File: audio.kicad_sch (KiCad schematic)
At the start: 59 parts, among them IC1 TAC5212IRGER, J13 Headphones 3.5mm, J16 Debug, J18 Jack 6.35mm, J19 Jack 6.35mm, J20 Jack 6.35mm, J22 Jack 6.35mm, U14 OPA1656ID, U7 74AHCT1G32SE-7

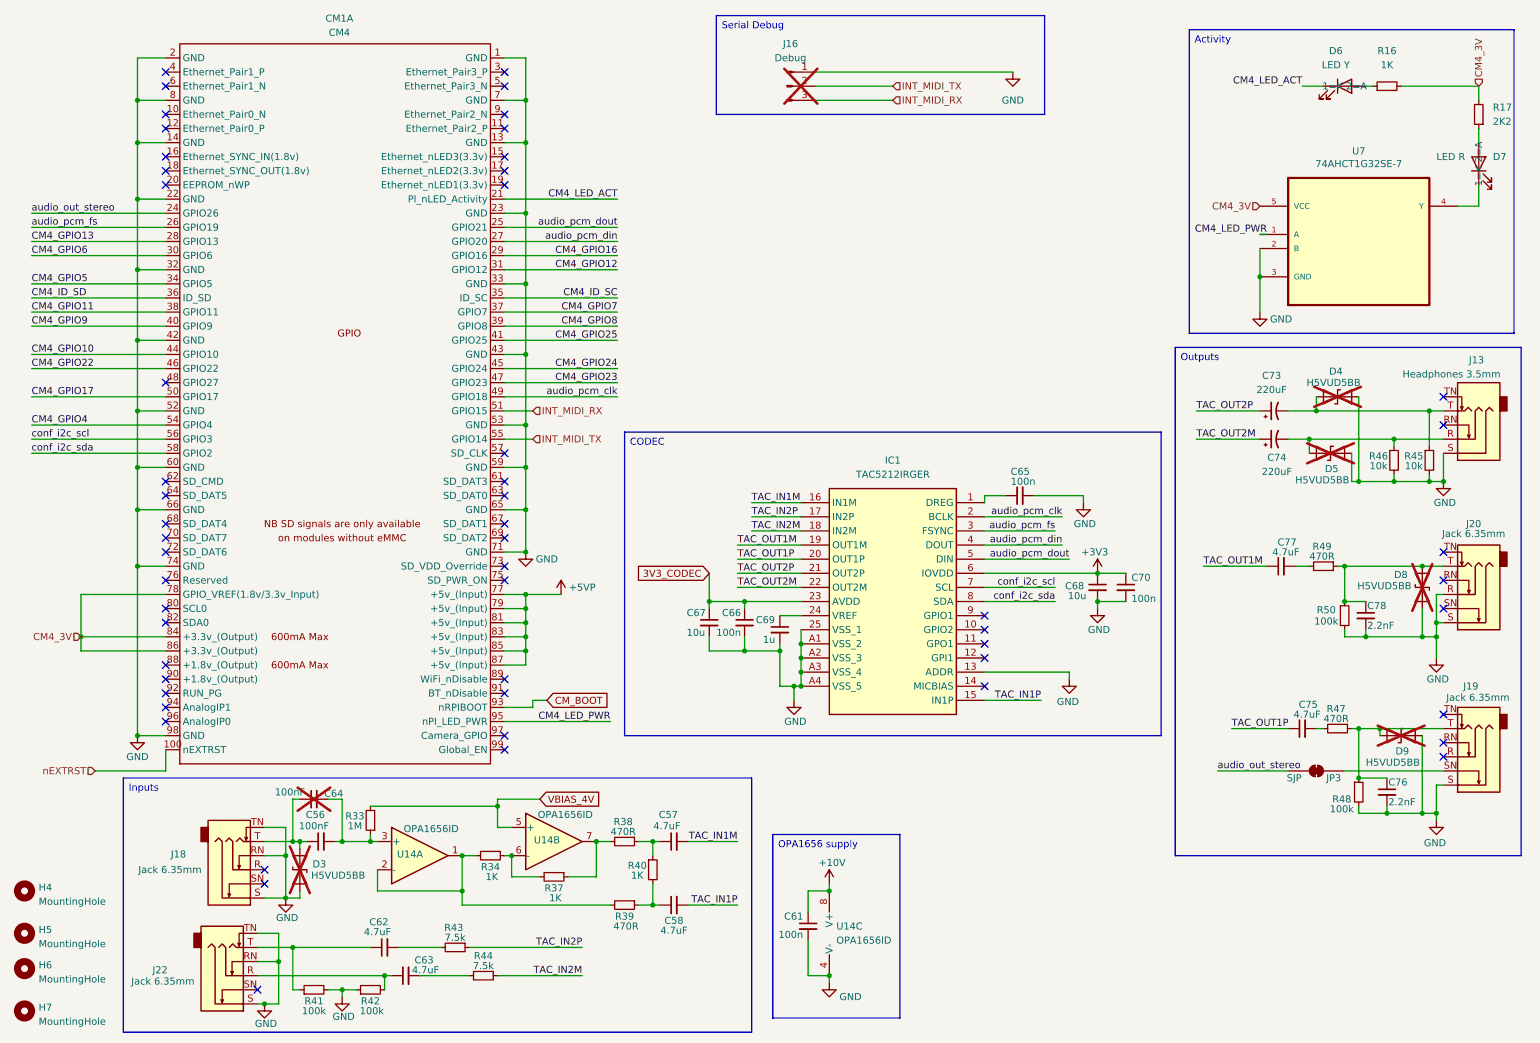
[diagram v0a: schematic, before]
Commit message: Changed to CM5, removed unnecessary USB chips, Changing RP2024 to STM32.
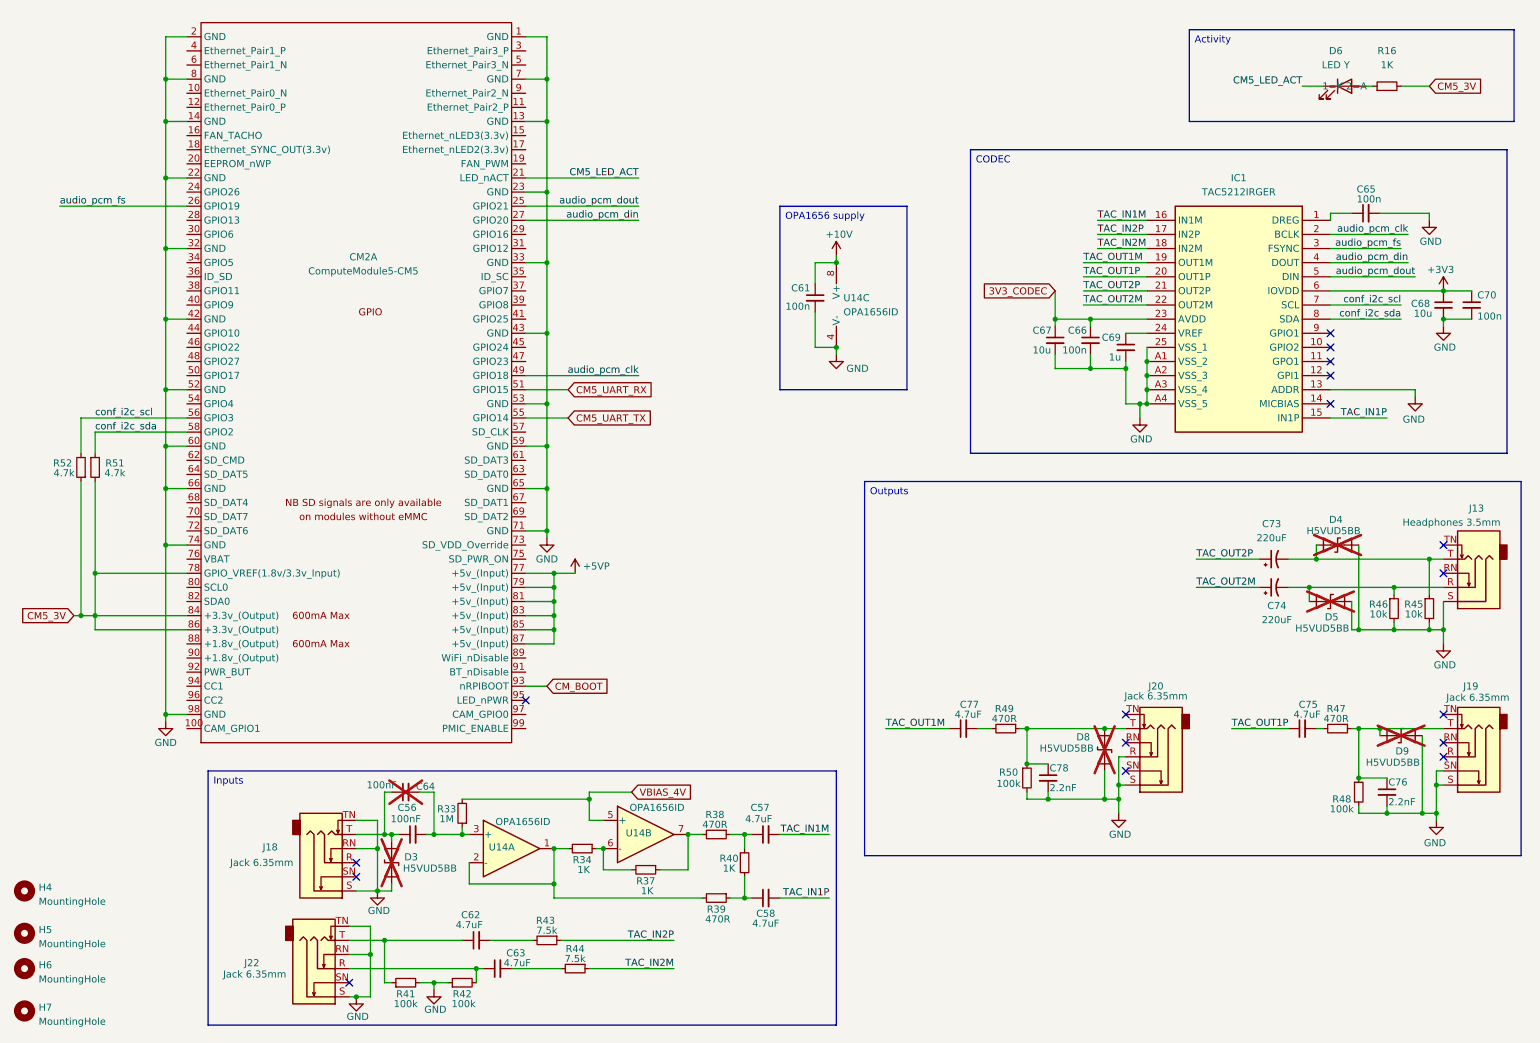
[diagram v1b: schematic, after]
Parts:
- removed CM1: CM4, Pedalboard Library:Raspberry-Pi-4-Compute-Module, symbol pedalboard:CM4
- removed D7: LED R, LED_SMD:LED_0805_2012Metric, symbol Device:LED
- removed J16: Debug, Connector_PinHeader_2.54mm:PinHeader_1x03_P2.54mm_Vertical, symbol Connector:Conn_01x03_Pin
- removed JP3: SJP, symbol Jumper:SolderJumper_2_Bridged
- removed R17: 2K2, Resistor_SMD:R_0805_2012Metric, symbol Device:R_Small
- removed U7: 74AHCT1G32SE-7, Package_TO_SOT_SMD:SOT-353_SC-70-5, symbol pedalboard:74AHCT1G32SE-7
- added CM2: ComputeModule5-CM5, CM5IO:Raspberry-Pi-5-Compute-Module, symbol CM5IO:ComputeModule5-CM5
- added R51, R52: 4.7k, Resistor_SMD:R_0603_1608Metric, symbol Device:R_Small
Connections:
- net +5VP: now also CM2.77 (+5v_(Input)), CM2.79 (+5v_(Input)), CM2.81 (+5v_(Input)), CM2.83 (+5v_(Input)), CM2.85 (+5v_(Input)), CM2.87 (+5v_(Input))
- net CM_BOOT: now also CM2.93 (nRPIBOOT)
- net GND: now also J19.SN, CM2.1 (GND), CM2.13 (GND), CM2.14 (GND), CM2.2 (GND), CM2.22 (GND), CM2.23 (GND), CM2.32 (GND), CM2.33 (GND), CM2.42 (GND), CM2.43 (GND), CM2.52 (GND), CM2.53 (GND), CM2.59 (GND), CM2.60 (GND), CM2.65 (GND), CM2.66 (GND), CM2.7 (GND), CM2.71 (GND), CM2.74 (GND), CM2.8 (GND), CM2.98 (GND)
- net audio_pcm_clk: now also CM2.49 (GPIO18)
- net audio_pcm_din: now also CM2.27 (GPIO20)
- net audio_pcm_dout: now also CM2.25 (GPIO21)
- net audio_pcm_fs: now also CM2.26 (GPIO19)
- net conf_i2c_scl: now also CM2.56 (GPIO3), R52.2
- net conf_i2c_sda: now also CM2.58 (GPIO2), R51.1
- net CM4_3V renamed CM5_3V
- net CM5_3V: now also CM2.78 (GPIO_VREF(1.8v/3.3v_Input)), CM2.84 (+3.3v_(Output)), CM2.86 (+3.3v_(Output)), R51.2, R52.1
- net CM4_LED_ACT renamed CM5_LED_ACT
- net CM5_LED_ACT: now also CM2.21 (LED_nACT)
- new net CM5_UART_RX: CM2.51 (GPIO15)
- new net CM5_UART_TX: CM2.55 (GPIO14)
- no-connect marks 55 -> 17
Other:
- moved on the sheet: C56, C57, C58, C61, C62, C63, C64, C65, C66, C67, C68, C69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
